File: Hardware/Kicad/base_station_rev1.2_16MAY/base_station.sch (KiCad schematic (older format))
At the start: 86 parts, among them CON1 USB-MICRO-B, CON2 AVR-ISP-6, J1 RJ45-CON, P1 CONN_1, P2 CONN_1, P3 CONN_1, P4 CONN_1, Q1 MOS_N, SW1 SW_PUSH, U1 AP7333-33SAG-7, U2 ATMEGA32U4, U3 W5100, U4 RX2004A_BIW, U5 NRF24L01, U6 24AA02E48T-I/OT, X1 8MHz, X2 25MHz

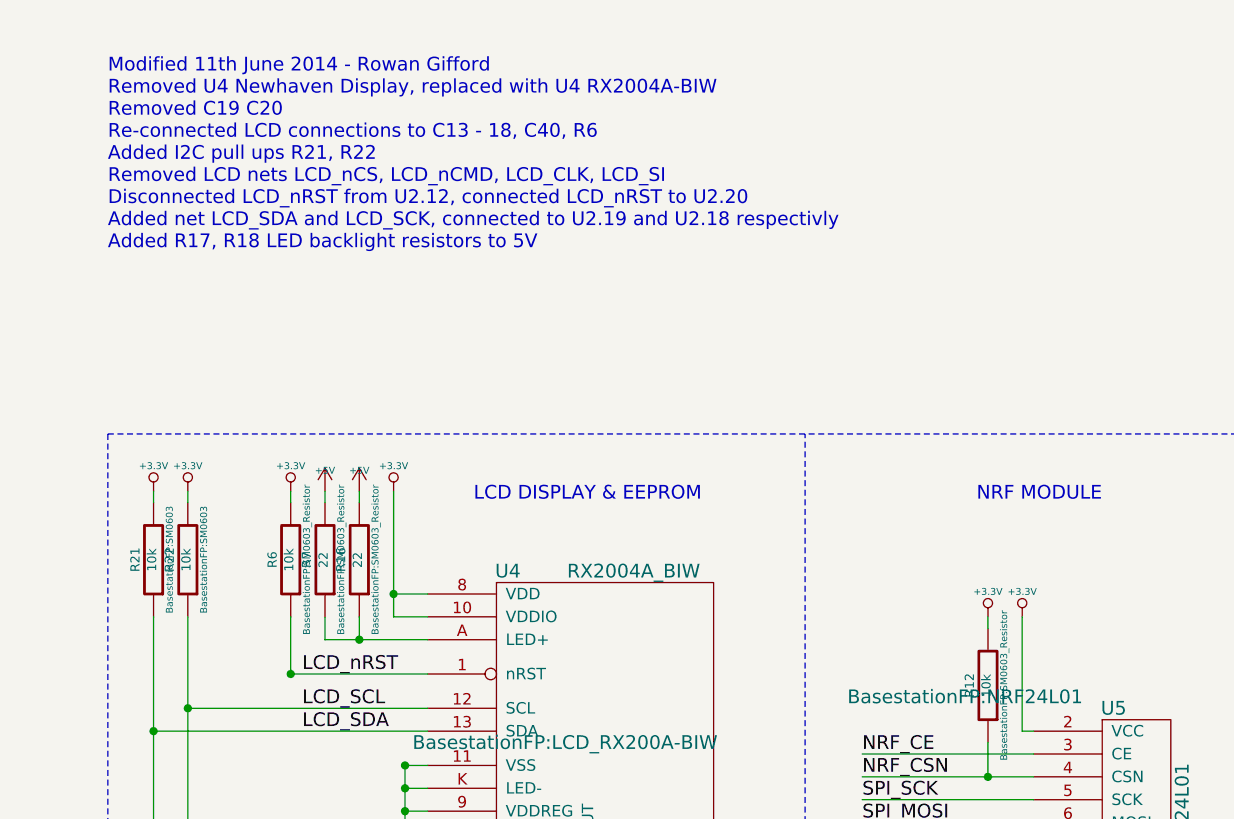
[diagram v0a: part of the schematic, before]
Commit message: Modified HW - BS gerbers
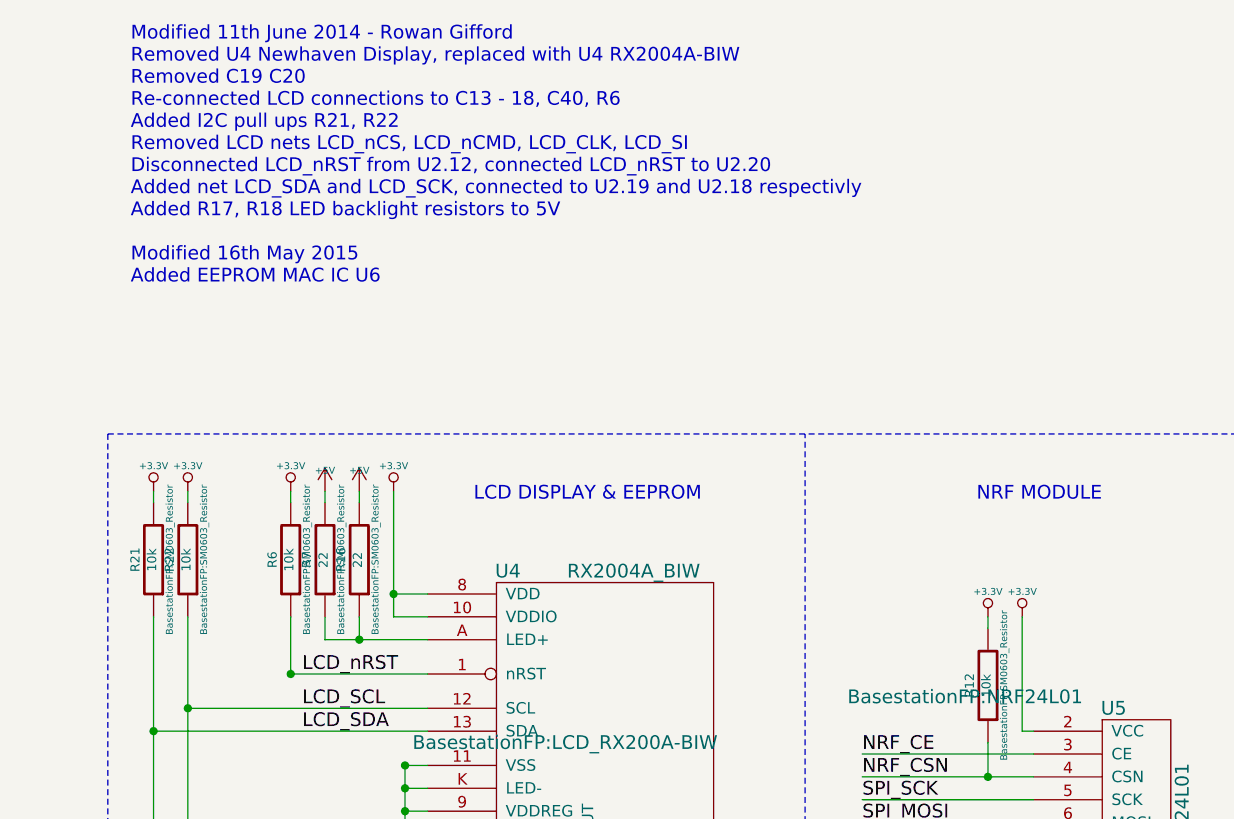
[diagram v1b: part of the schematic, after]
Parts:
- FID1, FID2, FID3: footprint (none) -> BasestationFP:Fiducial
- R21, R22: footprint BasestationFP:SM0603 -> BasestationFP:SM0603_Resistor
